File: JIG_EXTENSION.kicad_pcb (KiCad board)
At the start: 2 copper layers, 180 x 180 mm, 114 parts, among them J1 Conn_01x03_Pin, J10 USB_B, J11 VIN, J12 Conn_01x02_Pin, J13 Conn_01x02_Pin, J14 Conn_01x02_Pin, J15 Conn_01x02_Pin, J16 Conn_01x02_Pin, J17 VIN, J18 Conn_01x04_Pin, J19 Conn_01x04_Pin, J20 Conn_01x04_Pin, J21 VIN, J22 Conn_02x04_Odd_Even, J3 Conn_01x07_Pin, J4 Conn_01x12_Socket, J5 Conn_01x12_Socket, J6 VIN, J7 618037231321, J8 Conn_01x18_Pin, J9 Conn_01x19_Pin, Q1 WST3325, U1 ESP32-DEVKIT-V1, U10 MCP2562-E-MF, U11 MAX13487EESAT, U2 CH340E, U3 AMS1117-3.3, U4 NCP1117DT50RKG, U5 SN74LVC1G3157DBVR, U6 SN74LVC1G3157DBVR, U9 MCP2515-xST, Y1 16MHz

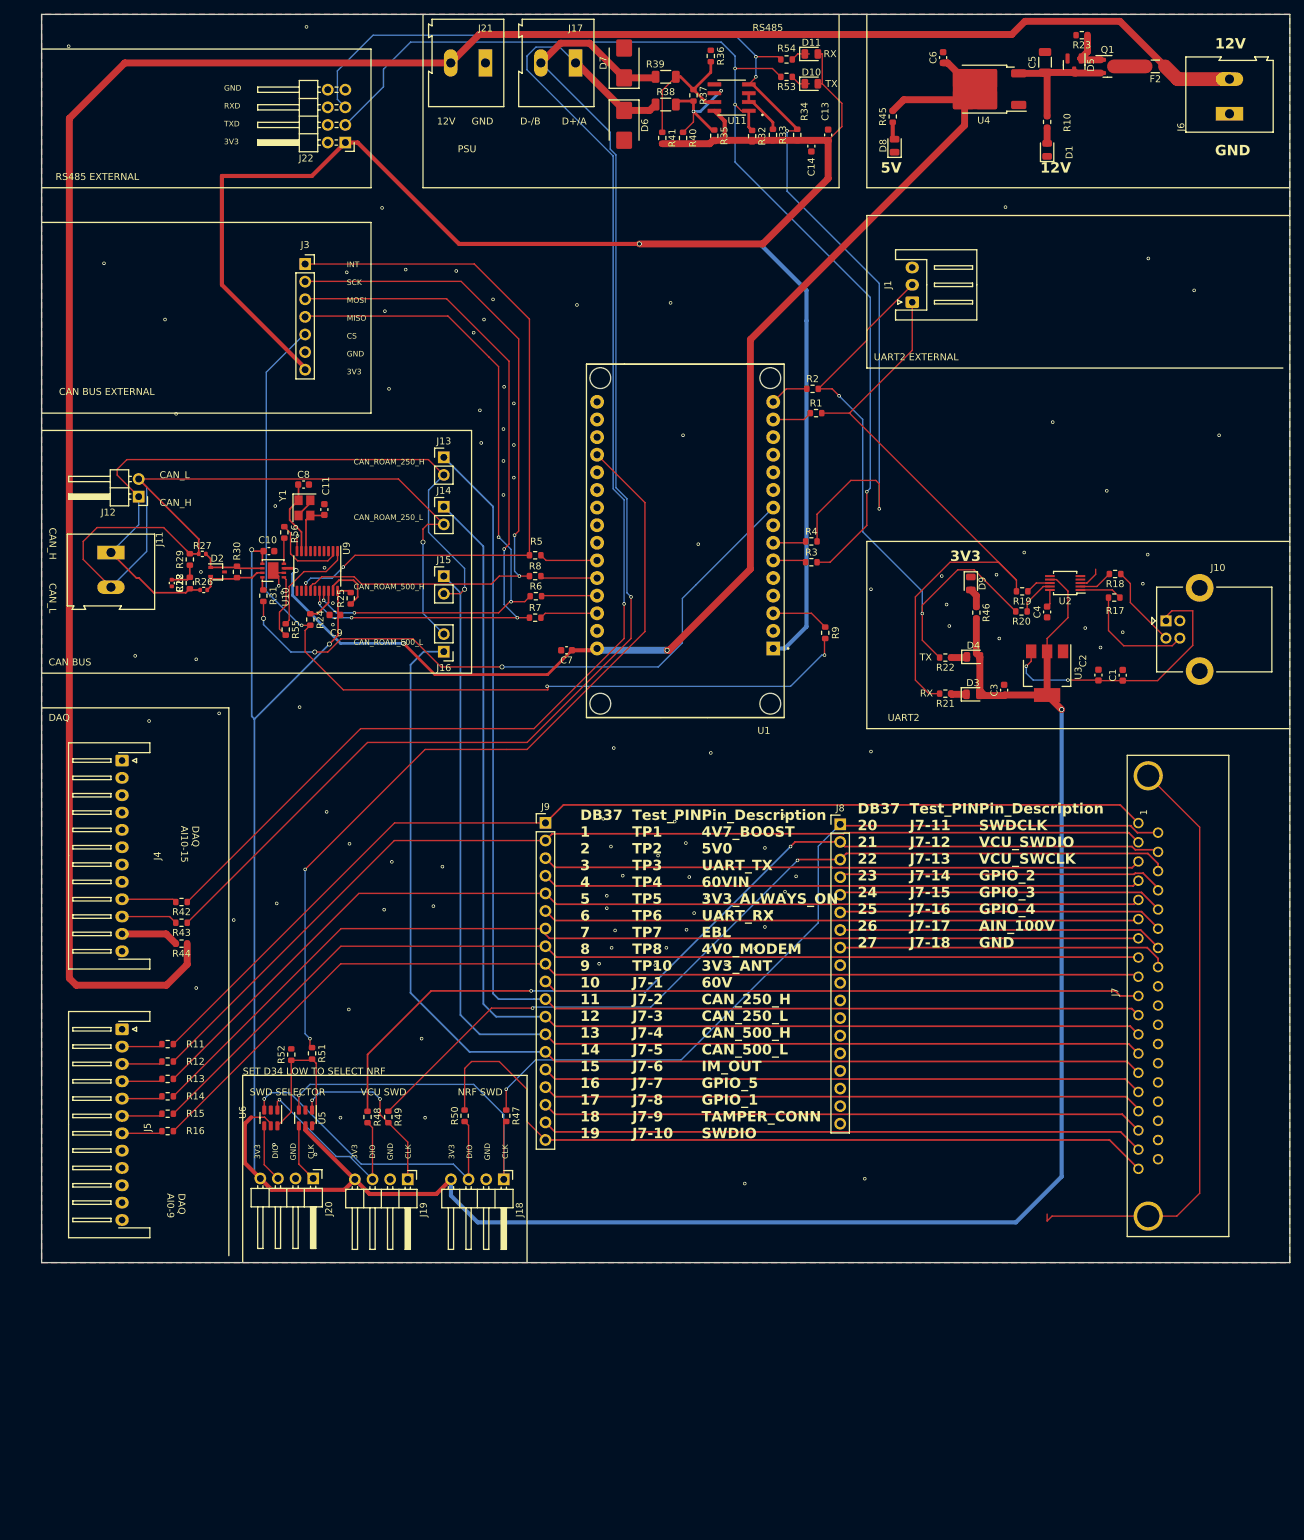
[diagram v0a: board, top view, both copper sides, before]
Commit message: done
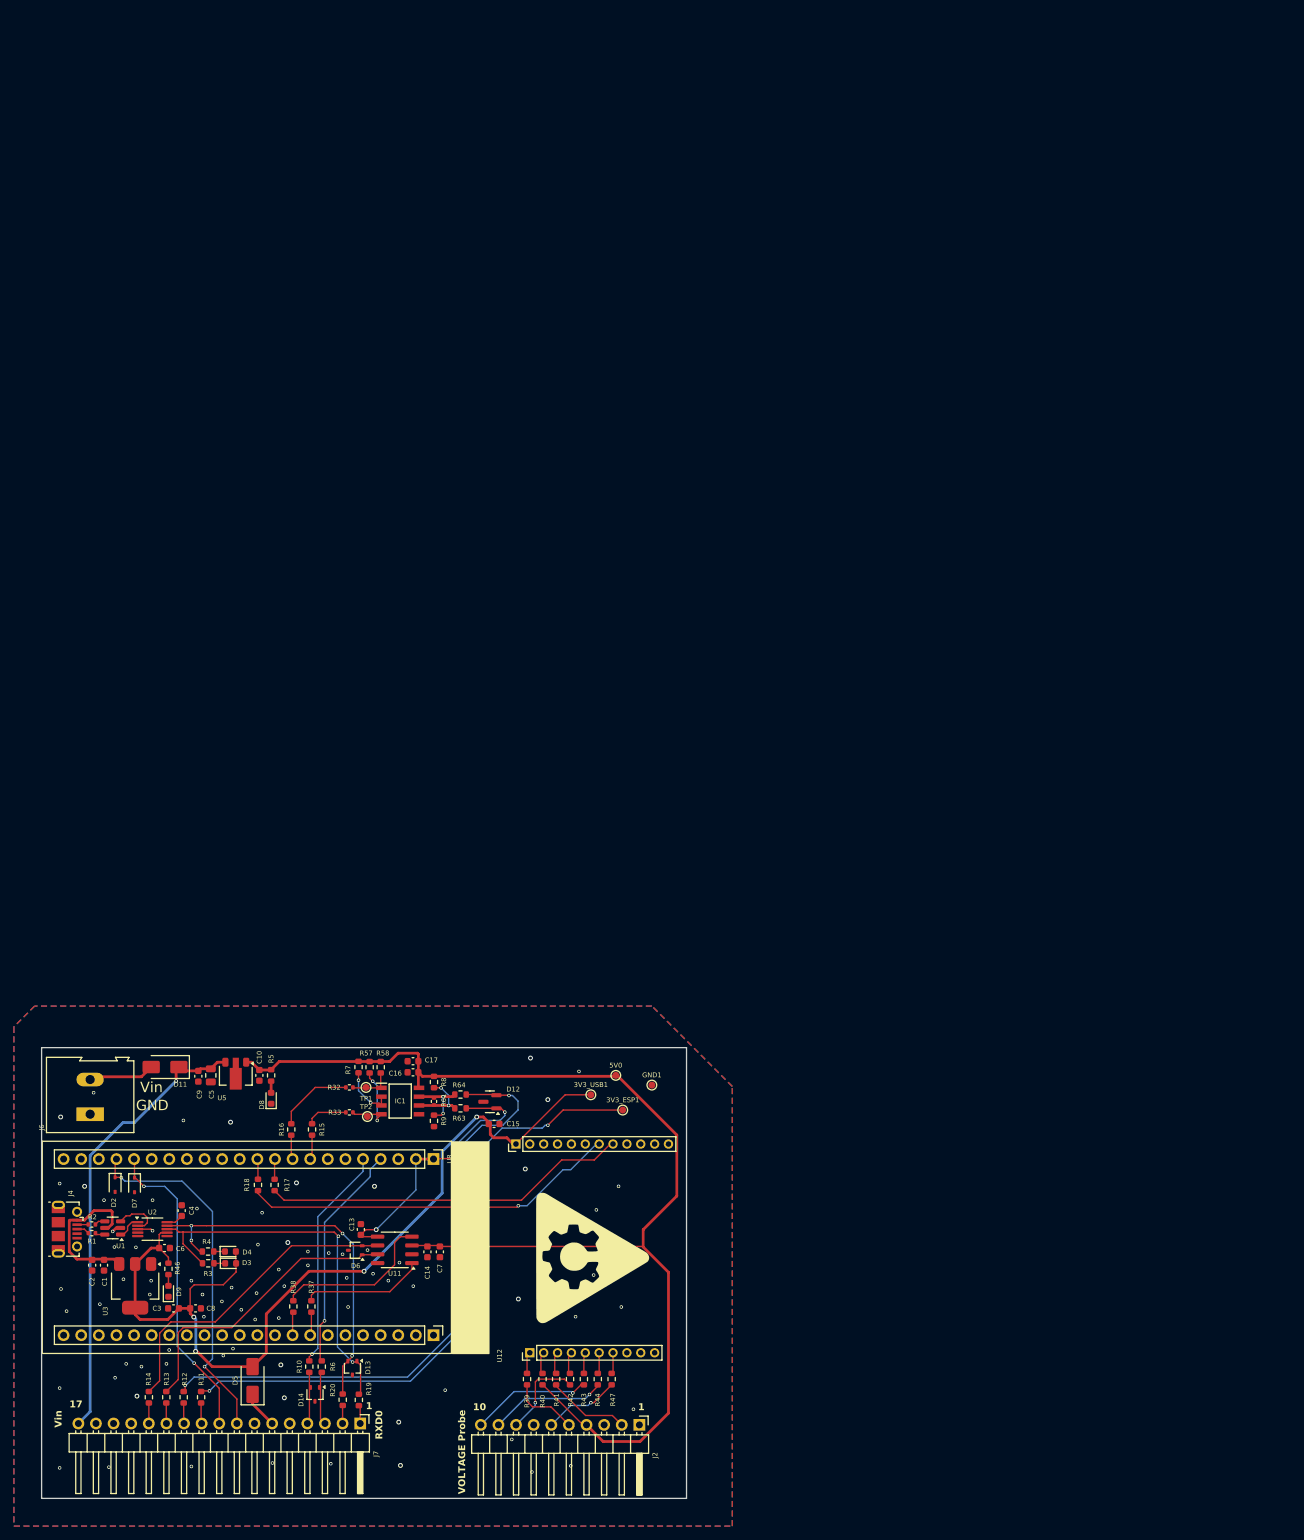
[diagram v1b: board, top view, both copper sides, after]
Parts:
- removed C11: 18pF, Capacitor_SMD:C_0603_1608Metric
- removed C12: 1nF, Capacitor_SMD:C_0402_1005Metric
- removed D1, D10: LED, LED_SMD:LED_0805_2012Metric
- removed F2: C1F 2, Fuse:Fuse_1206_3216Metric
- removed J1: Conn_01x03_Pin, Connector_JST:JST_XH_S3B-XH-A_1x03_P2.50mm_Horizontal
- removed J10: USB_B, Connector_USB:USB_B_Lumberg_2411_02_Horizontal
- removed J11, J17, J21: VIN, TerminalBlock:TerminalBlock_Altech_AK300-2_P5.00mm
- removed J12: Conn_01x02_Pin, Connector_PinHeader_2.54mm:PinHeader_1x02_P2.54mm_Horizontal
- removed J13, J14, J15, J16: Conn_01x02_Pin, Connector_PinHeader_2.54mm:PinHeader_1x02_P2.54mm_Vertical
- removed J18, J19, J20: Conn_01x04_Pin, Connector_PinHeader_2.54mm:PinHeader_1x04_P2.54mm_Horizontal
- removed J22: Conn_02x04_Odd_Even, Connector_PinHeader_2.54mm:PinHeader_2x04_P2.54mm_Horizontal
- removed J3: Conn_01x07_Pin, Connector_PinSocket_2.54mm:PinSocket_1x07_P2.54mm_Vertical
- removed J5: Conn_01x12_Socket, Connector_JST:JST_XH_S12B-XH-A-1_1x12_P2.50mm_Horizontal
- removed J8: Conn_01x18_Pin, Connector_PinHeader_2.54mm:PinHeader_1x18_P2.54mm_Vertical
- removed J9: Conn_01x19_Pin, Connector_PinHeader_2.54mm:PinHeader_1x19_P2.54mm_Vertical
- removed Q1: WST3325, Package_TO_SOT_SMD:SOT-23
- removed R21, R22, R53, R54: 1K, Resistor_SMD:R_0603_1608Metric
- removed R23: 100k, Resistor_SMD:R_0603_1608Metric
- removed R24, R25, R34: 10k, Resistor_SMD:R_0603_1608Metric
- removed R26, R27: 0, Resistor_SMD:R_0402_1005Metric
- removed R28, R29: 2k8, Resistor_SMD:R_0603_1608Metric
- removed R30: DNP, Resistor_SMD:R_0603_1608Metric
- removed R31, R48, R49, R50, R51, R55, R56: 0, Resistor_SMD:R_0603_1608Metric
- removed R35, R36: 4k7, Resistor_SMD:R_0603_1608Metric
- removed R45: 2k, Resistor_SMD:R_0603_1608Metric
- removed R52: 10K, Resistor_SMD:R_0603_1608Metric
- removed U10: MCP2562-E-MF, Package_DFN_QFN:DFN-8-1EP_3x3mm_P0.65mm_EP1.55x2.4mm
- removed U4: NCP1117DT50RKG, Package_TO_SOT_SMD:TO-252-2
- removed U6: SN74LVC1G3157DBVR, Package_TO_SOT_SMD:SOT-23-6
- removed U9: MCP2515-xST, Package_SO:TSSOP-20_4.4x6.5mm_P0.65mm
- removed Y1: 16MHz, Crystal:Crystal_SMD_Abracon_ABM8G-4Pin_3.2x2.5mm
- added 3V3_ESP1: TP_V, TestPoint:TestPoint_Pad_D1.0mm, F.Cu at (245.6, 184.9)
- added 3V3_USB1: TP_V, TestPoint:TestPoint_Pad_D1.0mm, F.Cu at (241.0, 182.7)
- added 5V0: TP_V, TestPoint:TestPoint_Pad_D1.0mm, F.Cu at (244.6, 179.9)
- added C15: 10uF, Capacitor_SMD:C_0603_1608Metric, F.Cu at (227.1, 186.9)
- added C16: 100nF, Capacitor_SMD:C_0603_1608Metric, F.Cu at (215.4, 179.5)
- added C17: 1uF, Capacitor_SMD:C_0603_1608Metric, F.Cu at (215.4, 177.9)
- added D12: PESD8V0L2BT-N, Package_TO_SOT_SMD:SOT-23, F.Cu at (226.4, 183.8)
- added D13: SM712_SOT23, Package_TO_SOT_SMD:SOT-323_SC-70, F.Cu at (206.6, 222.1)
- added D14: SM712_SOT23, Package_TO_SOT_SMD:SOT-323_SC-70, F.Cu at (201.2, 225.9)
- added G***: LOGO, LOGO, F.Cu at (240.0, 205.9)
- added GND1: TP_V, TestPoint:TestPoint_Pad_D1.0mm, F.Cu at (249.8, 181.3)
- added IC1: MAX13487EESA+T, YZ-ICs:SOIC127P600X175-8N, F.Cu at (213.5, 183.6)
- added J2: Conn_01x10_Pin, Connector_PinHeader_2.54mm:PinHeader_1x10_P2.54mm_Horizontal, F.Cu at (248.0, 230.3)
- added R57: 10K, Resistor_SMD:R_0603_1608Metric, F.Cu at (209.1, 178.8)
- added R58: 10K, Resistor_SMD:R_0603_1608Metric, F.Cu at (210.7, 178.8)
- added R61: DNP, Resistor_SMD:R_0402_1005Metric, F.Cu at (218.4, 183.7)
- added R63: 10, Resistor_SMD:R_0603_1608Metric, F.Cu at (222.2, 184.7)
- added R64: 10, Resistor_SMD:R_0603_1608Metric, F.Cu at (222.2, 182.7)
- added TP1: rs485_tx, TestPoint:TestPoint_Pad_D1.0mm, F.Cu at (208.6, 181.7)
- added TP2: rs485_tx, TestPoint:TestPoint_Pad_D1.0mm, F.Cu at (208.8, 185.9)
- added U12: K10-3U8S16D, YZ-Connector:K10-3U8S16D, F.Cu at (232.2, 219.9)
- added U8: ESP32-S3-WROOM-1_Devkit, YZ-Connector:ESP32S3_DevkitPinHeader_1x22_P2.54mm_Vertical, F.Cu at (218.3, 192.0)
- C1, C13, C4: value 100n -> 100nF
- C14: value 1u -> 100nF
- C2, C3: value 1u -> 1uF
- C5: value 10uF -> 0.33uF; footprint Capacitor_SMD:C_1206_3216Metric -> Capacitor_SMD:C_0805_2012Metric
- C6: value 10uF -> 100nF
- C8: value 18pF -> 10uF
- D11: value LED -> SS14; footprint LED_SMD:LED_0805_2012Metric -> Diode_SMD:D_SMA
- D2: value SM712_SOT23 -> 3V3_Z; footprint Package_TO_SOT_SMD:SOT-323_SC-70 -> Diode_SMD:D_SOD-323
- D3, D4, D8, D9: footprint LED_SMD:LED_0805_2012Metric -> LED_SMD:LED_0603_1608Metric
- D5: value BZX84B4V7LT1 -> SS14; footprint Package_TO_SOT_SMD:SOT-23 -> Diode_SMD:D_SMA
- D6: value 6.8V CA -> SM712_SOT23; footprint Diode_SMD:D_SMB -> Package_TO_SOT_SMD:SOT-323_SC-70
- D7: value 6.8V CA -> 3V3_Z; footprint Diode_SMD:D_SMB -> Diode_SMD:D_SOD-323
- J4: value Conn_01x12_Socket -> USB_B_Micro; footprint Connector_JST:JST_XH_S12B-XH-A-1_1x12_P2.50mm_Horizontal -> Connector_USB:USB_Micro-B_Molex-105017-0001
- J7: value 618037231321 -> Conn_01x17_Pin; footprint footprint:618037231321 -> Connector_PinHeader_2.54mm:PinHeader_1x17_P2.54mm_Horizontal
- R1, R2: value 0 -> 22; footprint Resistor_SMD:R_0603_1608Metric -> Resistor_SMD:R_0402_1005Metric
- R10: value 5k -> 0
- R3, R4, R5, R7, R8, R9: value 0 -> 4K7
- R32, R33: value 10k -> 22; footprint Resistor_SMD:R_0603_1608Metric -> Resistor_SMD:R_0402_1005Metric
- R37, R40, R41: value DNP -> 0
- R38, R39: value 10 -> 0; footprint Resistor_SMD:R_1206_3216Metric -> Resistor_SMD:R_0603_1608Metric
- R46: value 1K -> 4K7
- U1: value ESP32-DEVKIT-V1 -> USBLC6-2SC6; footprint footprint:MODULE_ESP32_DEVKIT_V1 -> Package_TO_SOT_SMD:SOT-23-6
- U11: value MAX13487EESAT -> TJA1051T/3; footprint footprint:SOIC127P600X175-8N -> Package_SO:SOIC-8_3.9x4.9mm_P1.27mm
- U5: value SN74LVC1G3157DBVR -> L78L05_SOT89; footprint Package_TO_SOT_SMD:SOT-23-6 -> Package_TO_SOT_SMD:SOT-89-3
- moved D5 223.7 mm to (192.2, 223.9), turned to 90 degrees
- moved J6 218.6 mm to (168.8, 185.5)
- moved R10 208.7 mm to (200.4, 221.9)
- moved C6 205.1 mm to (179.5, 204.8), turned to 0 degrees
- moved C5 189.3 mm to (186.2, 179.9), turned to -90 degrees
- moved R39 188.9 mm to (231.8, 223.7), turned to 90 degrees
- moved R37 183.1 mm to (200.7, 213.3), turned to 90 degrees
- moved R38 181.5 mm to (198.1, 213.3), turned to 90 degrees
- moved R40 180.1 mm to (234.0, 223.7), turned to 90 degrees
- moved R41 179.6 mm to (236.0, 223.7), turned to 90 degrees
- moved D7 176.5 mm to (175.2, 195.7), turned to -90 degrees
- moved D11 173.3 mm to (179.6, 178.7), turned to 180 degrees
- moved U11 173.1 mm to (212.7, 205.1)
- moved C13 171.6 mm to (207.8, 202.2), turned to -90 degrees
- moved C1 169.8 mm to (170.8, 207.3), turned to -90 degrees
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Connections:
- C1 pad 1: Net-(J10-VBUS) -> /USB_VBUS
- C10 pad 1: GND -> 5V0
- C10 pad 2: 3V3_B -> GND
- C13 pad 1: 3V3 -> GND
- C13 pad 2: GND -> 3V3_OUT_ESP
- C14 pad 1: 3V3 -> GND
- C14 pad 2: GND -> 5V0
- C2 pad 1: Net-(J10-VBUS) -> /USB_VBUS
- C5 pad 1: Net-(D5-K) -> 12V
- C6 pad 1: 5V0 -> 3V3_B
- C8 pad 1: /CAN_OSC_1 -> 3V3_B
- C9 pad 1: GND -> 12V
- C9 pad 2: 3V3_B -> GND
- D11 pad 1: Net-(D11-K) -> 12V
- D11 pad 2: 3V3 -> Net-(D11-A)
- D2 pad 1: Net-(D2-A1) -> /IGN
- D2 pad 2: Net-(D2-A2) -> GND
- D5 pad 1: Net-(D5-A) -> /VBAT
- D5 pad 2: (no net) -> 3V3_B
- D6 pad 1: /D+/A -> /CAN_500_H
- D6 pad 2: GND -> /CAN_500_L
- D7 pad 1: /D-/B -> /IM
- J4 pad 1: GND -> /USB_VBUS
- J4 pad 2: /AI10 -> Net-(J4-D-)
- J4 pad 3: /AI11 -> Net-(J4-D+)
- J4 pad 4: /AI12 -> unconnected-(J4-ID-Pad4)
- J4 pad 5: /AI13 -> GND
- J4 pad 6: /AI14 -> GND
- J6 pad 2: +12V -> Net-(D11-A)
- J7 pad 1: /DB_1 -> /RXD0
- J7 pad 10: /DB_10 -> /D-
- J7 pad 11: /DB_11 -> /D+
- J7 pad 12: /DB_12 -> /C_H
- J7 pad 13: /DB_13 -> /C_L
- J7 pad 14: /DB_14 -> /IO_E
- J7 pad 15: /DB_15 -> /ADC_I
- J7 pad 16: /DB_16 -> GND
- J7 pad 17: /DB_17 -> 12V
- J7 pad 2: /DB_2 -> /TXD0
- J7 pad 3: /DB_3 -> /EN
- J7 pad 4: /DB_4 -> /IO0
- J7 pad 5: /DB_5 -> /NTC
- J7 pad 6: /DB_6 -> /VBAT
- J7 pad 7: /DB_7 -> GND
- J7 pad 8: /DB_8 -> /IGN
- J7 pad 9: /DB_9 -> /IM
- R1 pad 1: Net-(U1-D22) -> Net-(R1-Pad1)
- R1 pad 2: /UART_QT_RX -> Net-(J4-D+)
- R10 pad 1: Net-(D1-A) -> /IO0
- R10 pad 2: Net-(D5-K) -> Net-(U8-IO5)
- R11 pad 1: /AI0 -> /D-
- R11 pad 2: /DB_1 -> /D-/B
- R12 pad 1: /AI1 -> /D+
- R12 pad 2: /DB_2 -> /D+/A
- R13 pad 1: /AI2 -> /C_H
- R13 pad 2: /DB_5 -> /CAN_500_H
- R14 pad 1: /AI3 -> /C_L
- R14 pad 2: /DB_7 -> /CAN_500_L
- R15 pad 1: /AI4 -> /RS485_TX
- R15 pad 2: /DB_8 -> Net-(R15-Pad2)
- R16 pad 1: /AI5 -> /RS485_RX
- R16 pad 2: /DB_9 -> Net-(U8-IO16)
- R17 pad 1: Net-(J10-D+) -> /K10_TX
- R17 pad 2: Net-(U2-UD+) -> Net-(U8-IO17)
- R18 pad 1: Net-(J10-D-) -> /K10_RX
- R18 pad 2: Net-(U2-UD-) -> Net-(U8-IO18)
- R19 pad 1: Net-(U2-TXD) -> /RXD0
- R19 pad 2: /UART_QT_RX -> /CH340_TX
- R2 pad 1: Net-(U1-D23) -> Net-(R2-Pad1)
- R2 pad 2: /UART_QT_TX -> Net-(J4-D-)
- R20 pad 1: Net-(U2-RXD) -> /TXD0
- R20 pad 2: /UART_QT_TX -> /CH340_RX
- R3 pad 1: /UART2_RX -> /CH340_TX
- R3 pad 2: /UART_RS485_TX -> Net-(D3-K)
- R32 pad 1: /UART_RS485_TX -> Net-(IC1-RO)
- R32 pad 2: 3V3 -> /RS485_RX
- R33 pad 1: Net-(U11-~{RE}) -> Net-(IC1-DI)
- R33 pad 2: 3V3 -> /RS485_TX
- R37 pad 1: Net-(U11-B) -> Net-(U8-IO40)
- R37 pad 2: Net-(U11-A) -> /CAN_TXD
- R38 pad 1: /D+/A -> Net-(U8-IO39)
- R38 pad 2: Net-(U11-A) -> /CAN_RXD
- R39 pad 1: /D-/B -> /5V0_BUCK
- R39 pad 2: Net-(U11-B) -> Net-(U12-AIN1)
- R4 pad 1: /UART2_TX -> /CH340_RX
- R4 pad 2: /UART_RS485_RX -> Net-(D4-K)
- R40 pad 1: Net-(U11-A) -> 5V0
- R40 pad 2: 3V3 -> Net-(U12-AIN2)
- R41 pad 1: Net-(U11-B) -> /3V3_AWS
- R41 pad 2: 3V3 -> Net-(U12-AIN3)
- R42 pad 1: /D+/A -> /4V0
- R42 pad 2: /A/D+ -> Net-(U12-AIN4)
- R43 pad 1: /D-/B -> /3V3_LDO
- R43 pad 2: /B/D- -> Net-(U12-AIN5)
- R44 pad 1: +12V -> /4V7_BOOST
- R44 pad 2: /+VS -> Net-(U12-AIN6)
- R47 pad 1: /DB_20 -> /3V3_ANT
- R47 pad 2: /SWCLK -> Net-(U12-AIN7)
- R5 pad 1: Net-(U1-D27) -> 5V0
- R5 pad 2: /CAN_INT -> Net-(D8-A)
- R6 pad 1: /MISO -> /EN
- R6 pad 2: Net-(U1-D12) -> Net-(U8-IO4)
- R7 pad 1: /MOSI -> Net-(IC1-~{RE})
- R7 pad 2: Net-(U1-D13) -> 5V0
- R8 pad 1: /SCK -> 5V0
- R8 pad 2: Net-(U1-D14) -> Net-(IC1-A)
- R9 pad 1: /CS -> Net-(IC1-B)
- R9 pad 2: Net-(U1-D15) -> GND
- U1 pad 1: 3V3 -> /USB_DP
- U1 pad 3: Net-(U1-D15) -> /USB_DM
- U1 pad 4: unconnected-(U1-D2-Pad4) -> Net-(R2-Pad1)
- U1 pad 5: unconnected-(U1-D4-Pad5) -> /USB_VBUS
- U1 pad 6: /UART2_RX -> Net-(R1-Pad1)
- U11 pad 1: /UART_RS485_TX -> /CAN_TXD
- U11 pad 2: Net-(U11-~{RE}) -> GND
- U11 pad 3: Net-(U11-~{RE}) -> 5V0
- U11 pad 4: /UART_RS485_RX -> /CAN_RXD
- U11 pad 5: GND -> 3V3_OUT_ESP
- U11 pad 6: Net-(U11-A) -> /CAN_500_L
- U11 pad 7: Net-(U11-B) -> /CAN_500_H
- U11 pad 8: 3V3 -> GND
- U2 pad 1: Net-(U2-UD+) -> /USB_DP
- U2 pad 2: Net-(U2-UD-) -> /USB_DM
- U2 pad 8: Net-(U2-TXD) -> /CH340_TX
- U2 pad 9: Net-(U2-RXD) -> /CH340_RX
- U3 pad 3: Net-(J10-VBUS) -> /USB_VBUS
- U5 pad 1: /VCU_SWCLK -> 5V0
- U5 pad 3: /SWCLK -> 12V
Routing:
- net +12V: track 322.2 -> 0.00 mm
- net 3V3: track 263.8 -> 0.00 mm, vias 1 -> 0
- net 3V3_B: track 381.7 -> 131.2 mm, vias 3 -> 4
- net /DB_11: track 174.6 -> 0.00 mm
- net /DB_12: track 170.3 -> 0.00 mm
- net /UART_RS485_RX: track 167.7 -> 0.00 mm, vias 4 -> 0
- net /DB_13: track 164.4 -> 0.00 mm
- net /DB_14: track 162.6 -> 0.00 mm
- net /UART_RS485_TX: track 161.8 -> 0.00 mm, vias 3 -> 0
- net /DB_1: track 154.5 -> 0.00 mm
- net /DB_2: track 153.4 -> 0.00 mm
- net /DB_5: track 151.1 -> 0.00 mm
- net /DB_7: track 150.2 -> 0.00 mm
- net /DB_9: track 150.0 -> 0.00 mm
- net /DB_8: track 149.8 -> 0.00 mm
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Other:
- board size 180 x 180 mm -> 93 x 65 mm
- board text added: "1"
- board text added: "10"
- board text added: "17"
- board text added: "RXD0"
- board text added: "VOLTAGE Probe"
- board text added: "Vin"
- board text removed: "12V"
- board text removed: "3V3"
- board text removed: "3V3 DIO GND CLK"
- board text removed: "5V"
- board text removed: "CAN BUS"
- board text removed: "CAN BUS EXTERNAL"
- board text removed: "CAN_H"
- board text removed: "CAN_L"
- board text removed: "CAN_ROAM_250_H"
- board text removed: "CAN_ROAM_250_L"
- board text removed: "CAN_ROAM_500_H"
- board text removed: "CAN_ROAM_500_L"
- board text removed: "D+/A"
- board text removed: "D-/B"
- board text removed: "DAQ"
- board text removed: "DAQ AI0-9"
- board text removed: "DAQ AI10-15"
- board text removed: "DB37 1 2 3 4 5 6 7 8 9 10 11 12 13 14 15 16 17 18 19"
- board text removed: "DB37 20 21 22 23 24 25 26 27"
- board text removed: "GND RXD TXD 3V3"
- board text removed: "INT SCK MOSI MISO CS GND 3V3"
- board text removed: "NRF SWD"
- board text removed: "PSU"
- board text removed: "Pin_Description 4V7_BOOST 5V0 UART_TX 60VIN 3V3_ALWAYS_ON UART_RX EBL 4V0_MODEM 3V3_ANT 60V CAN_250_H CAN_250_L CAN_500_H CAN_500_L IM_OUT GPIO_5 GPIO_1 TAMPER_CONN SWDIO"
- board text removed: "Pin_Description SWDCLK VCU_SWDIO VCU_SWCLK GPIO_2 GPIO_3 GPIO_4 AIN_100V GND"
- board text removed: "RS485"
- board text removed: "RS485 EXTERNAL"
- board text removed: "RX"
- board text removed: "SET D34 LOW TO SELECT NRF"
- board text removed: "SWD SELECTOR"
- board text removed: "TX"
- board text removed: "Test_PIN J7-11 J7-12 J7-13 J7-14 J7-15 J7-16 J7-17 J7-18"
- board text removed: "Test_PIN TP1 TP2 TP3 TP4 TP5 TP6 TP7 TP8 TP10 J7-1 J7-2 J7-3 J7-4 J7-5 J7-6 J7-7 J7-8 J7-9 J7-10"
- board text removed: "UART2"
- board text removed: "UART2 EXTERNAL"
- board text removed: "VCU SWD"
